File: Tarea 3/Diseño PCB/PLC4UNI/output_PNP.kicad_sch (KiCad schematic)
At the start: 0 parts

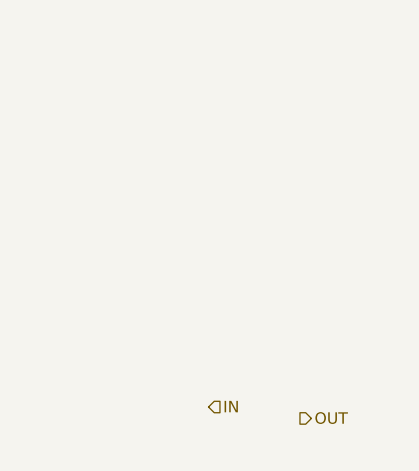
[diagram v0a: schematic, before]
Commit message: Tarea 3
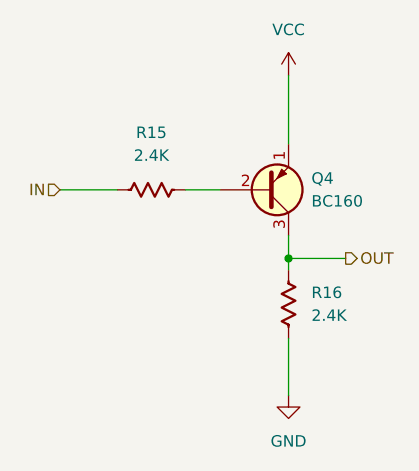
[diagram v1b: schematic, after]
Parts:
- added Q4: BC160, PCM_Package_TO_SOT_THT_AKL:TO-39-3_EBC, symbol PCM_Transistor_BJT_AKL:BC160
- added R15, R16: 2.4K, PCM_Resistor_SMD_AKL:R_0603_1608Metric, symbol PCM_Resistor_US_AKL:R_0603
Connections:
- net IN: now also R15.1
- net OUT: now also Q4.3 (C), R16.2
- new net: Q4.2 (B), R15.2
- new net GND: R16.1
- new net VCC: Q4.1 (E)

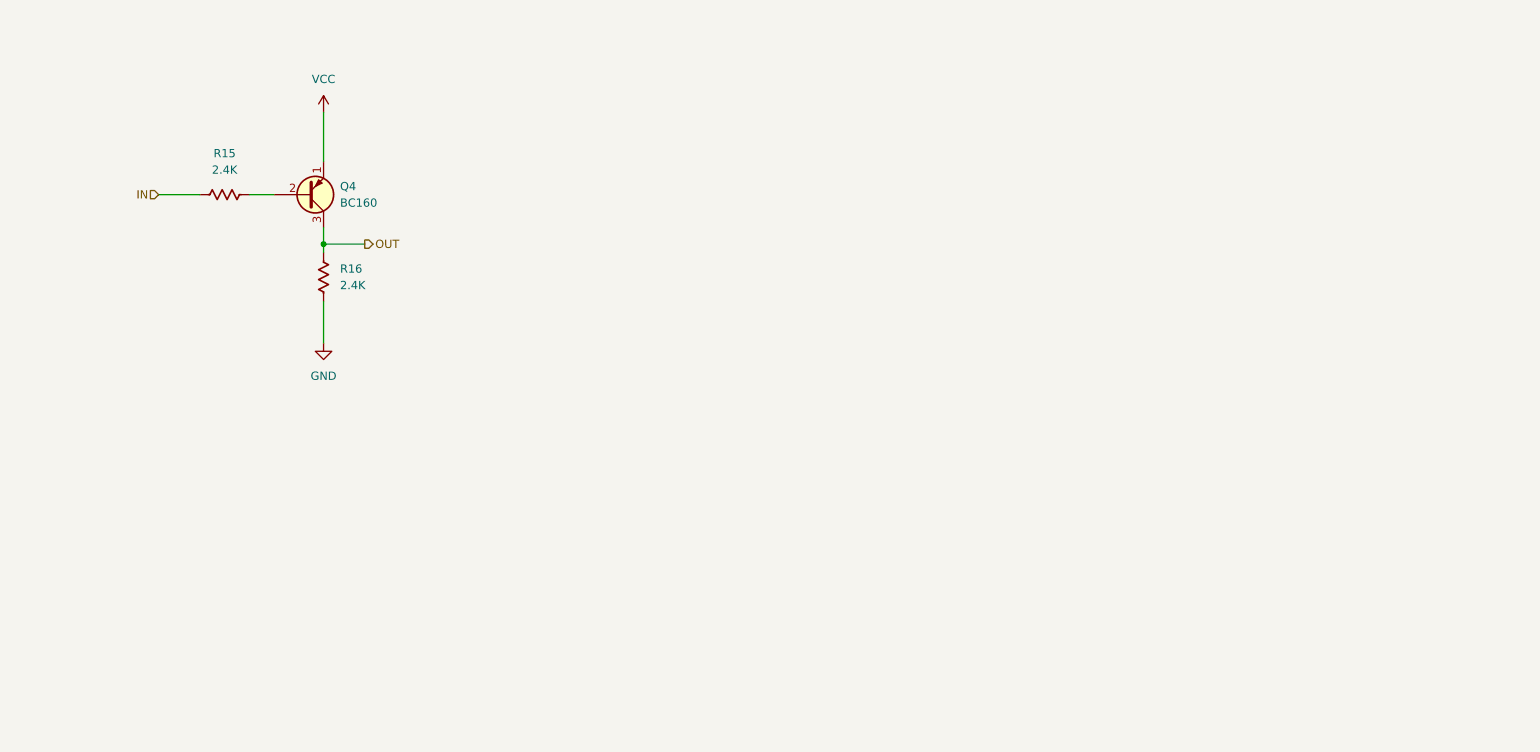
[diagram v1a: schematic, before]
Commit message: Tarea 3
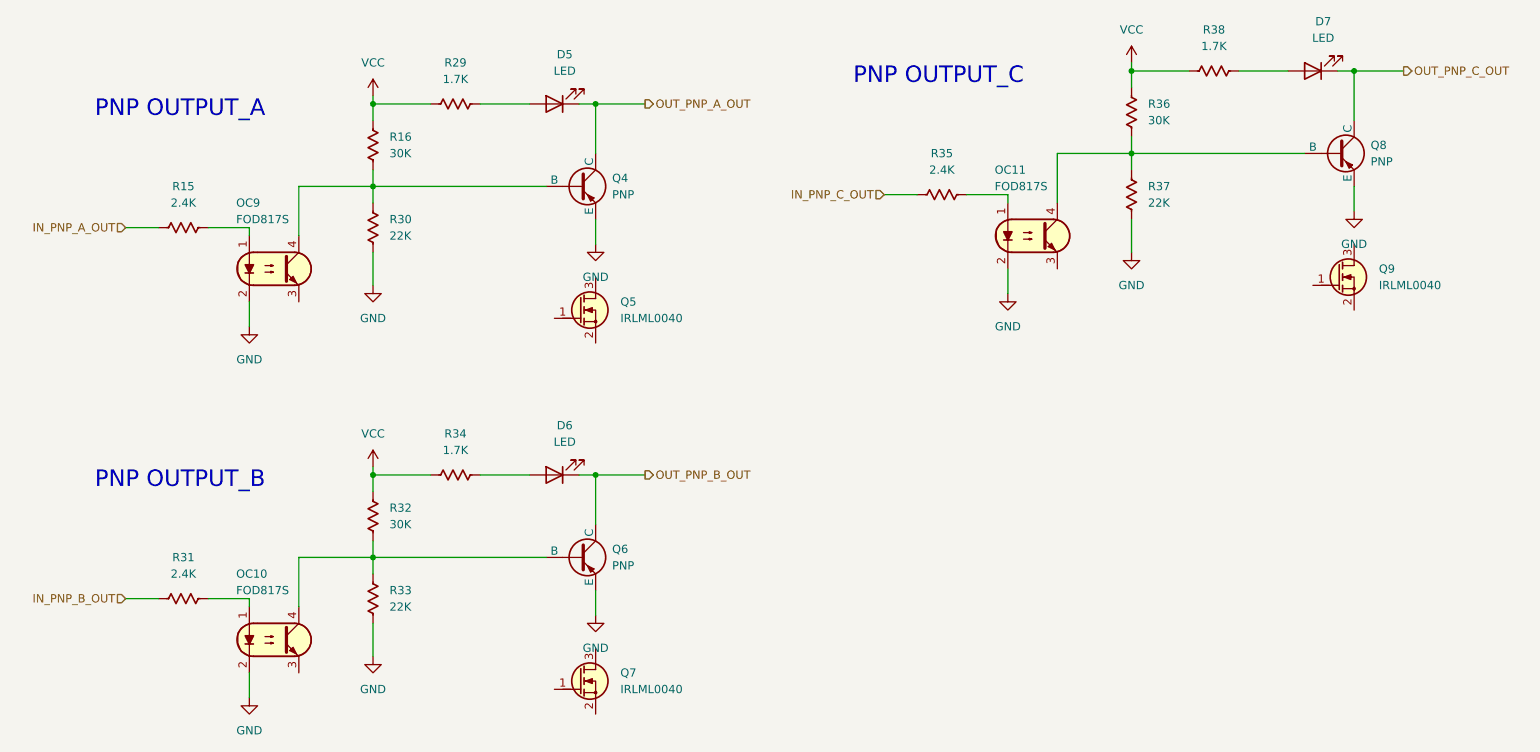
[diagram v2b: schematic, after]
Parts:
- removed Q4: BC160, PCM_Package_TO_SOT_THT_AKL:TO-39-3_EBC, symbol PCM_Transistor_BJT_AKL:BC160
- added D5, D6, D7: LED, symbol Device:LED
- added OC10, OC11, OC9: FOD817S, PCM_Package_DIP_AKL:SMDIP-4_W9.53mm, symbol PCM_Optocoupler_AKL:FOD817S
- added Q4, Q6, Q8: PNP, symbol Simulation_SPICE:PNP
- added Q5, Q7, Q9: IRLML0040, PCM_Package_TO_SOT_SMD_AKL:SOT-23, symbol PCM_Transistor_MOSFET_AKL:IRLML0040
- added R29, R34, R38: 1.7K, PCM_Resistor_SMD_AKL:R_0603_1608Metric, symbol PCM_Resistor_US_AKL:R_0603
- added R30, R33, R37: 22K, PCM_Resistor_SMD_AKL:R_0603_1608Metric, symbol PCM_Resistor_US_AKL:R_0603
- added R31, R35: 2.4K, PCM_Resistor_SMD_AKL:R_0603_1608Metric, symbol PCM_Resistor_US_AKL:R_0603
- added R32, R36: 30K, PCM_Resistor_SMD_AKL:R_0603_1608Metric, symbol PCM_Resistor_US_AKL:R_0603
- R16: value 2.4K -> 30K
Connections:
- net OUT is gone; now on net VCC: R16.2
- net GND: now also OC10.2, OC11.2, OC9.2, Q4.3 (E), Q6.3 (E), Q8.3 (E), R30.1, R33.1, R37.1; no longer R16.1
- net VCC: now also R29.2, R32.2, R34.2, R36.2, R38.2
- net at R15.2: now also OC9.1
- net IN renamed IN_PNP_A_OUT
- new net: D5.2 (A), R29.1
- new net: OC10.1, R31.2
- new net: OC10.4, Q6.2 (B), R32.1, R33.2
- new net: OC9.4, Q4.2 (B), R16.1, R30.2
- new net: D6.2 (A), R34.1
- new net: D7.2 (A), R38.1
- new net: OC11.1, R35.2
- new net: OC11.4, Q8.2 (B), R36.1, R37.2
- new net IN_PNP_B_OUT: R31.1
- new net IN_PNP_C_OUT: R35.1
- new net OUT_PNP_A_OUT: D5.1 (K), Q4.1 (C)
- new net OUT_PNP_B_OUT: D6.1 (K), Q6.1 (C)
- new net OUT_PNP_C_OUT: D7.1 (K), Q8.1 (C)
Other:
- note added: "PNP OUTPUT_A"
- note added: "PNP OUTPUT_B"
- note added: "PNP OUTPUT_C"
- moved on the sheet: R15, R16
